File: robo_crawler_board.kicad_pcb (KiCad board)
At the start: 2 copper layers, 26 parts, among them J1 Screw_Terminal_01x02, J2 Screw_Terminal_01x02, J3 Screw_Terminal_01x02, J4 Screw_Terminal_01x02, J5 Screw_Terminal_01x02, J6 Screw_Terminal_01x02, J7 Screw_Terminal_01x02, U4 DRV8871DDA, U5 DRV8871DDA, U6 DRV8871DDA, U7 DRV8871DDA, U8 DRV8871DDA, U9 DRV8871DDA

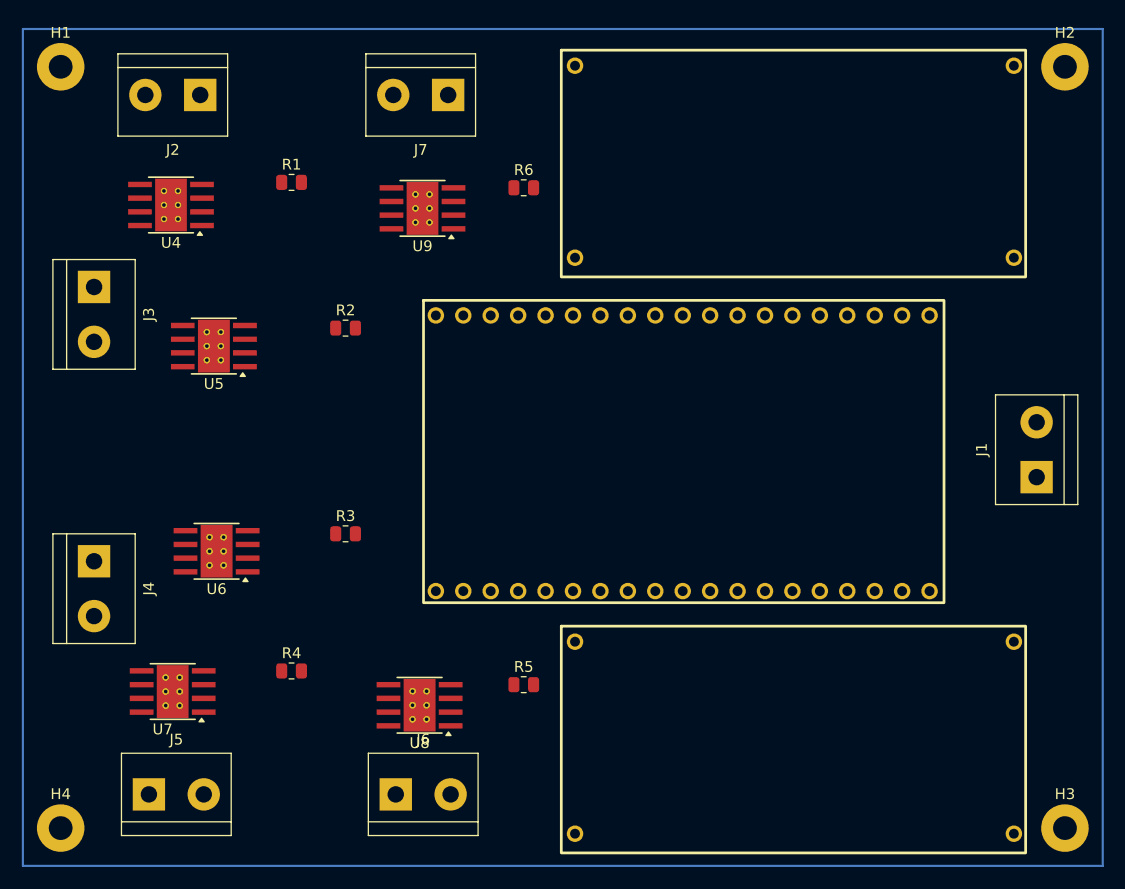
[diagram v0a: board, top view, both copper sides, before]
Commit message: tentative rev2
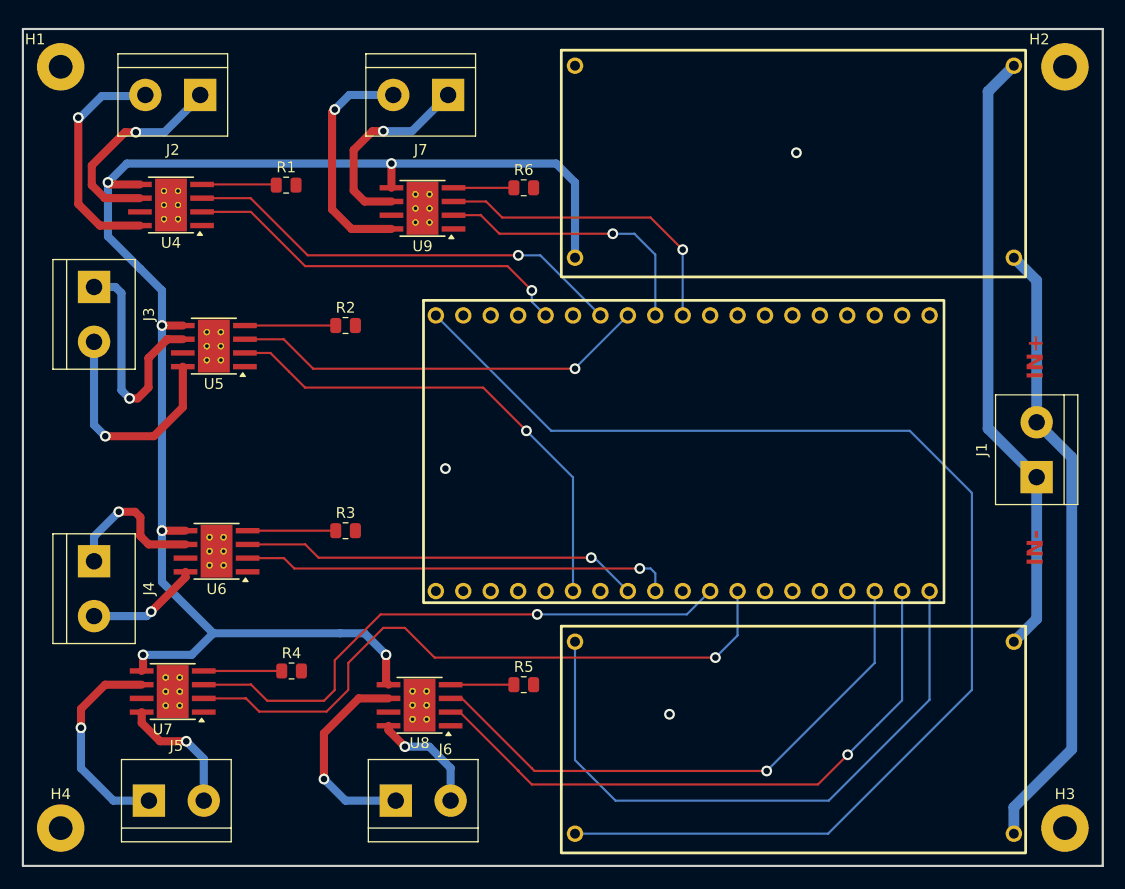
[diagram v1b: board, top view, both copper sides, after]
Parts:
- H1, H2, H4: value MountingHole -> M2
- moved J5 0.58 mm to (97.8, 122.5)
- moved J6 0.58 mm to (120.7, 122.5)
- moved R1 0.56 mm to (110.5, 65.5)
- moved R3 0.29 mm to (116.0, 97.5)
- moved R2 0.24 mm to (116.0, 78.5)
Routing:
- net +12V: track 0.00 -> 135.4 mm, vias 0 -> 6
- net +5V: track 0.00 -> 117.0 mm
- net MOTOR4_CH2: track 0.00 -> 60.7 mm, vias 0 -> 1
- net GND: track 0.00 -> 59.3 mm, vias 0 -> 3
- net MOTOR5_CH2: track 0.00 -> 57.9 mm, vias 0 -> 1
- net Net-(J1-Pin_2): track 0.00 -> 57.8 mm
- net Net-(J1-Pin_1): track 0.00 -> 57.1 mm
- net MOTOR4_CH1: track 0.00 -> 53.3 mm, vias 0 -> 1
- net MOTOR5_CH1: track 0.00 -> 52.9 mm, vias 0 -> 1
- net MOTOR2_CH2: track 0.00 -> 45.7 mm, vias 0 -> 1
- net MOTOR1_CH1: track 0.00 -> 41.4 mm, vias 0 -> 1
- net MOTOR3_CH2: track 0.00 -> 40.0 mm, vias 0 -> 1
- net MOTOR2_CH1: track 0.00 -> 38.7 mm, vias 0 -> 1
- net MOTOR3_CH1: track 0.00 -> 37.0 mm, vias 0 -> 1
- net MOTOR1_CH2: track 0.00 -> 36.4 mm, vias 0 -> 1
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- added copper zone on B.Cu, net GND
- added copper zone on F.Cu, net GND
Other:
- board outline added: 100 x 77.5 mm
- board text added: "IN+"
- board text added: "IN-"
